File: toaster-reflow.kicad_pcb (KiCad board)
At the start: 2 copper layers, 41.9 x 63.5 mm, 40 parts, among them J1 1935161, J2 1935161, J3 Raspberry_Pi_2_3, J4 1935161, J5 1935161, J6 Conn_01x03, K1 1-1415899-3, Q1 Q_PMOS_GSD, Q2 Q_PMOS_GSD, Q3 Q_PMOS_GSD, Q4 Q_PMOS_GSD, Q5 Q_PMOS_GSD, U1 3.3V Ref, U2 MAX31856, U3 MAX31856

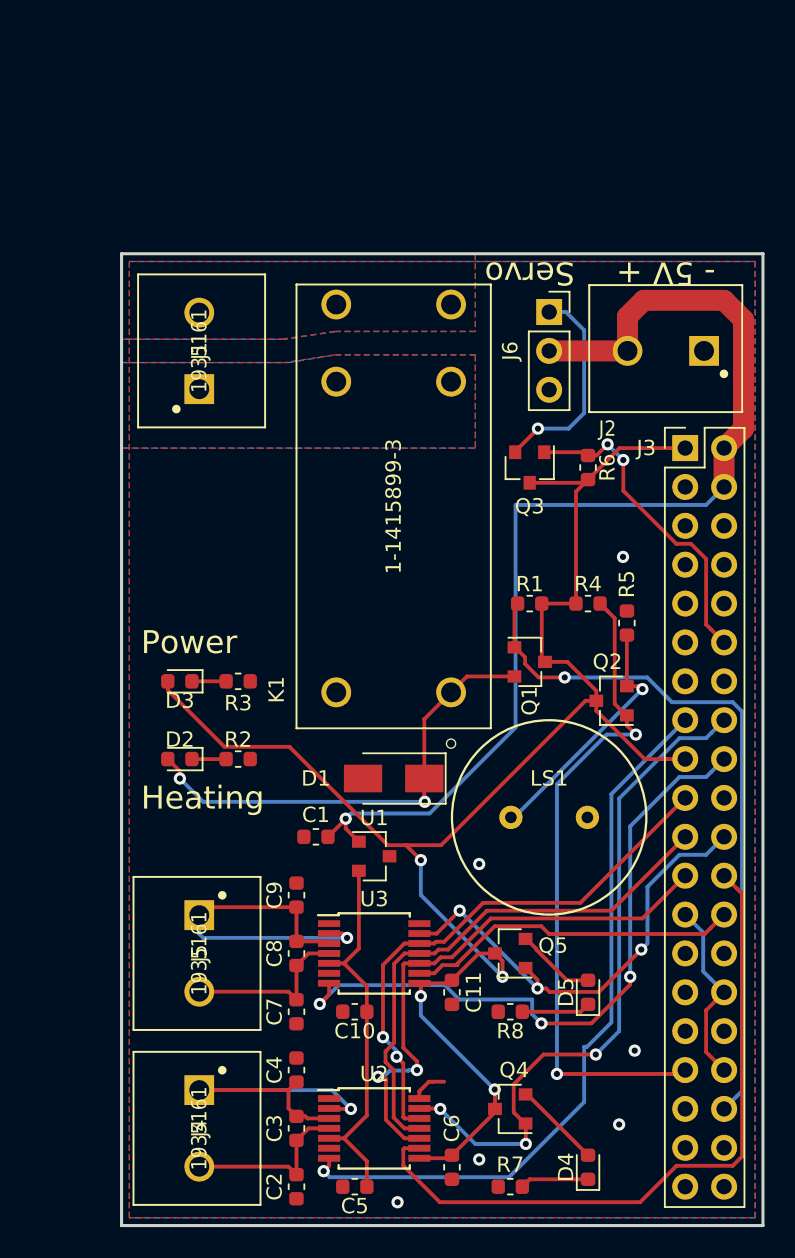
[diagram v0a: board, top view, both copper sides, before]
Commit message: Add a bunch of stuff
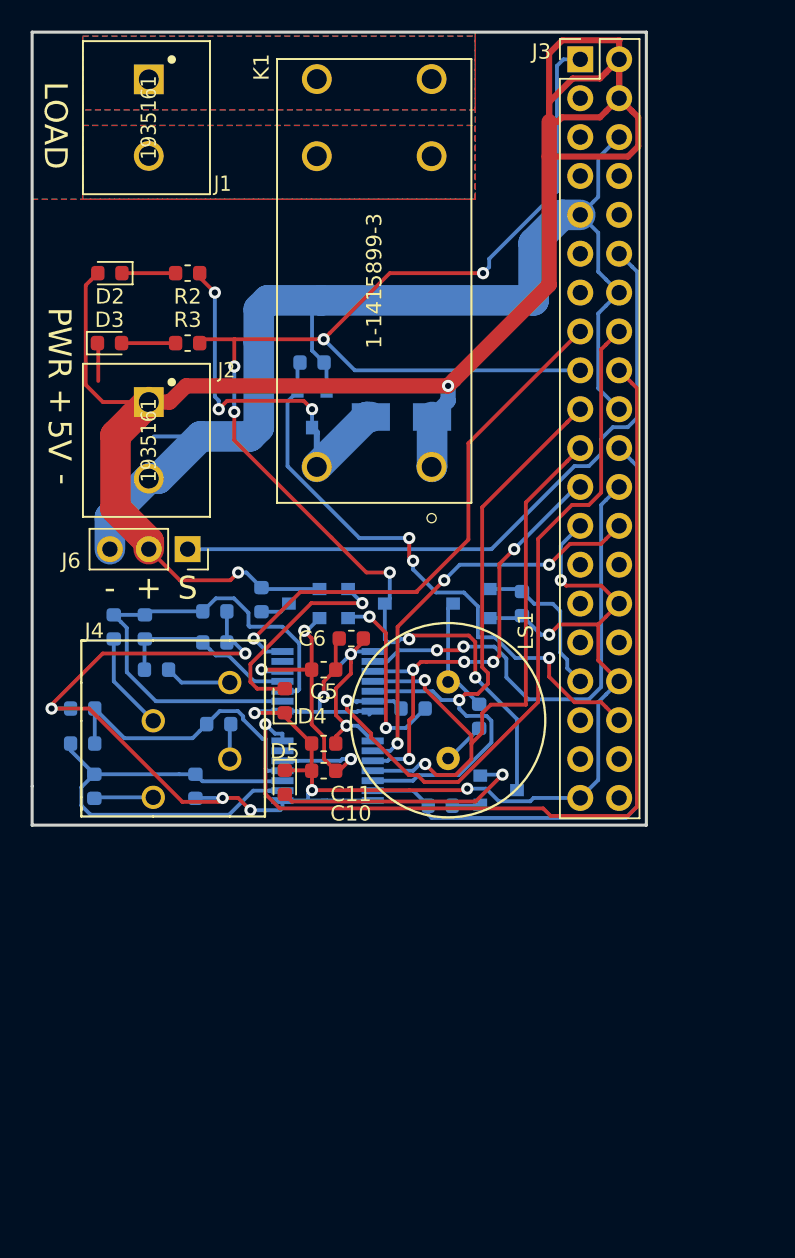
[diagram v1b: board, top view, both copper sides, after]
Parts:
- removed J5: 1935161, 1935161:PHOENIX_1935161
- removed Q5: Q_PMOS_GSD, Package_TO_SOT_SMD:SOT-23
- added R10: 100, Resistor_SMD:R_0603_1608Metric, B.Cu at (125.2, 122.4)
- added R11: 47k, Resistor_SMD:R_0603_1608Metric, B.Cu at (147.8, 123.7)
- added R9: 100, Resistor_SMD:R_0603_1608Metric, B.Cu at (133.3, 118.4)
- C1, C2, C3, C4, C7, C8, C9, D1, R1, R4, R5, U1, U2, U3: moved to B.Cu
- J4: value 1935161 -> Conn_01x04; footprint 1935161:PHOENIX_1935161 -> 1990025:1990025
- Q1, Q2: value Q_PMOS_GSD -> Q_NMOS_GSD; footprint Package_TO_SOT_SMD:SOT-23 -> Package_TO_SOT_SMD:SC-59; moved to B.Cu
- Q3, Q4: value Q_PMOS_GSD -> Q_PNP_BEC; footprint Package_TO_SOT_SMD:SOT-23 -> Package_TO_SOT_SMD:SC-59; moved to B.Cu
- R2: value 470 -> 1K
- R6: value 10K -> 100; moved to B.Cu
- R7: value 470 -> 100; moved to B.Cu
- R8: value 470 -> 47k; moved to B.Cu
- moved R7 44.8 mm to (126.5, 112.0), turned to 270 degrees
- moved D4 36.4 mm to (137.7, 116.8)
- moved C2 36.0 mm to (133.1, 113.0), turned to 180 degrees
- moved C6 35.2 mm to (142.0, 112.8), turned to 180 degrees
- moved J2 34.3 mm to (128.8, 99.8), turned to 270 degrees
- moved C3 34.2 mm to (128.5, 112.0)
- moved C5 33.8 mm to (140.2, 114.8), turned to 180 degrees
- moved D2 32.1 mm to (126.2, 88.9)
- moved R2 31.9 mm to (131.3, 88.9)
- moved R6 31.1 mm to (129.3, 114.8), turned to 0 degrees
- moved C4 30.4 mm to (133.1, 111.0), turned to 0 degrees
- moved U2 29.4 mm to (140.5, 115.6)
- moved J6 28.3 mm to (131.3, 106.9), turned to 270 degrees
- moved J3 26.3 mm to (157.0, 74.9)
- moved C7 24.2 mm to (124.5, 117.3), turned to 0 degrees
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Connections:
- D1 pad 1: Net-(D1-Pad1) -> +5V
- D1 pad 2: GND -> Net-(D1-Pad2)
- D2 pad 2: Net-(D1-Pad1) -> +5V
- D3 pad 1: Net-(D3-Pad1) -> GND
- D3 pad 2: +3V3 -> Net-(D3-Pad2)
- D4 pad 1: Net-(D4-Pad1) -> GND
- D5 pad 1: Net-(D5-Pad1) -> GND
- J2 pad 1: GND -> +5V
- J2 pad 2: +5V -> GND
- J4 pad 1: Net-(C3-Pad2) -> /Thermocouple2/T-
- J4 pad 2: Net-(C2-Pad2) -> /Thermocouple2/T+
- J6 pad 1: Net-(J6-Pad1) -> /SERVO_PWM
- K1 pad 11_1: Net-(J1-Pad1) -> Net-(J1-Pad2)
- K1 pad 11_2: Net-(J1-Pad1) -> Net-(J1-Pad2)
- K1 pad 14_1: Net-(J1-Pad2) -> Net-(J1-Pad1)
- K1 pad 14_2: Net-(J1-Pad2) -> Net-(J1-Pad1)
- K1 pad A1: Net-(D1-Pad1) -> +5V
- K1 pad A2: GND -> Net-(D1-Pad2)
- LS1 pad 2: GND -> Net-(LS1-Pad2)
- Q1 pad 2: Net-(D1-Pad1) -> GND
- Q1 pad 3: +3V3 -> Net-(D1-Pad2)
- Q2 pad 2: Net-(LS1-Pad1) -> GND
- Q2 pad 3: +3V3 -> Net-(LS1-Pad2)
- Q3 pad 1: /SERVO_PWM -> Net-(Q3-Pad1)
- Q3 pad 2: Net-(J6-Pad1) -> Net-(D4-Pad2)
- Q4 pad 1: /THERMO1_FAULT -> Net-(Q4-Pad1)
- Q4 pad 2: Net-(D4-Pad2) -> Net-(D5-Pad2)
- R1 pad 1: +3V3 -> /HEAT_ENABLE
- R1 pad 2: /HEAT_ENABLE -> GND
- R2 pad 1: GND -> Net-(D1-Pad2)
- R3 pad 1: GND -> Net-(D3-Pad2)
- R3 pad 2: Net-(D3-Pad1) -> +3V3
- R4 pad 1: +3V3 -> /BUZZER
- R4 pad 2: /BUZZER -> GND
- R5 pad 2: GND -> Net-(LS1-Pad2)
- R6 pad 1: +3V3 -> Net-(C2-Pad2)
- R6 pad 2: /SERVO_PWM -> /Thermocouple1/T+
- R7 pad 1: GND -> Net-(C3-Pad2)
- R7 pad 2: Net-(D4-Pad1) -> /Thermocouple1/T-
- R8 pad 1: GND -> Net-(Q3-Pad1)
- R8 pad 2: Net-(D5-Pad1) -> /THERMO1_FAULT
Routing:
- net GND: track 14.5 -> 202.0 mm, vias 6 -> 10
- net +5V: track 73.1 -> 119.5 mm, vias 1 -> 2
- net /BUZZER: track 43.5 -> 10.3 mm, vias 2 -> 0
- net Net-(D1-Pad1): track 30.7 -> 0.00 mm, vias 2 -> 0
- net Net-(D1-Pad2): track 0.00 -> 24.7 mm, vias 0 -> 3
- net /SERVO_PWM: track 21.2 -> 44.7 mm, vias 2 -> 0
- net /THERMO2_DRDY: track 43.3 -> 60.5 mm, vias 3 -> 1
- net /THERMO1_CS: track 45.3 -> 31.4 mm, vias 0 -> 2
- net Net-(J6-Pad1): track 13.8 -> 0.00 mm, vias 1 -> 0
- net Net-(LS1-Pad1): track 16.5 -> 2.85 mm, vias 1 -> 0
- net /THERMO1_DRDY: track 48.0 -> 35.6 mm
- net Net-(Q3-Pad1): track 0.00 -> 12.3 mm, vias 0 -> 2
- net /THERMO2_FAULT: track 30.8 -> 42.6 mm, vias 3 -> 0
- net Net-(D5-Pad2): track 5.23 -> 16.6 mm, vias 0 -> 1
- net Net-(C3-Pad2): track 22.5 -> 33.5 mm, vias 1 -> 0
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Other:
- board size 41.9 x 63.5 mm -> 40.1 x 51.8 mm
- board text added: "+"
- board text added: "-"
- board text added: "5V"
- board text added: "LOAD"
- board text added: "PWR"
- board text added: "S"
- board text removed: "- 5V +"
- board text removed: "Heating"
- board text removed: "Power"
- board text removed: "Servo"
